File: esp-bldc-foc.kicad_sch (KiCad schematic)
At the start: 8 parts, among them J10 UART, J7 A, J8 B, J9 C

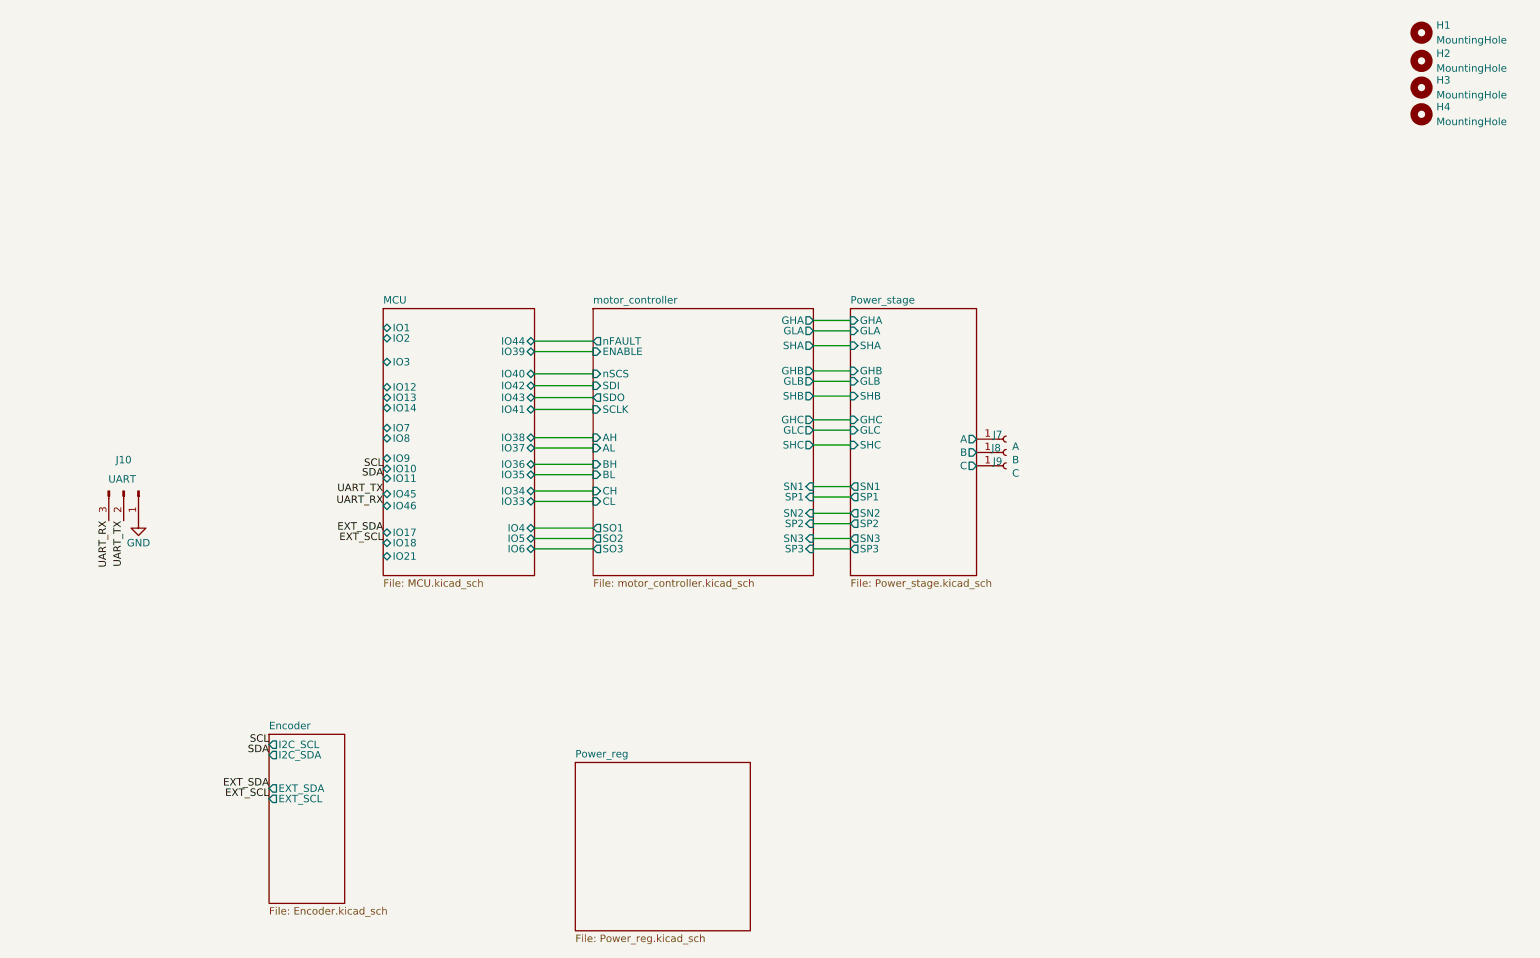
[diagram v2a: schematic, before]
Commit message: init routing done
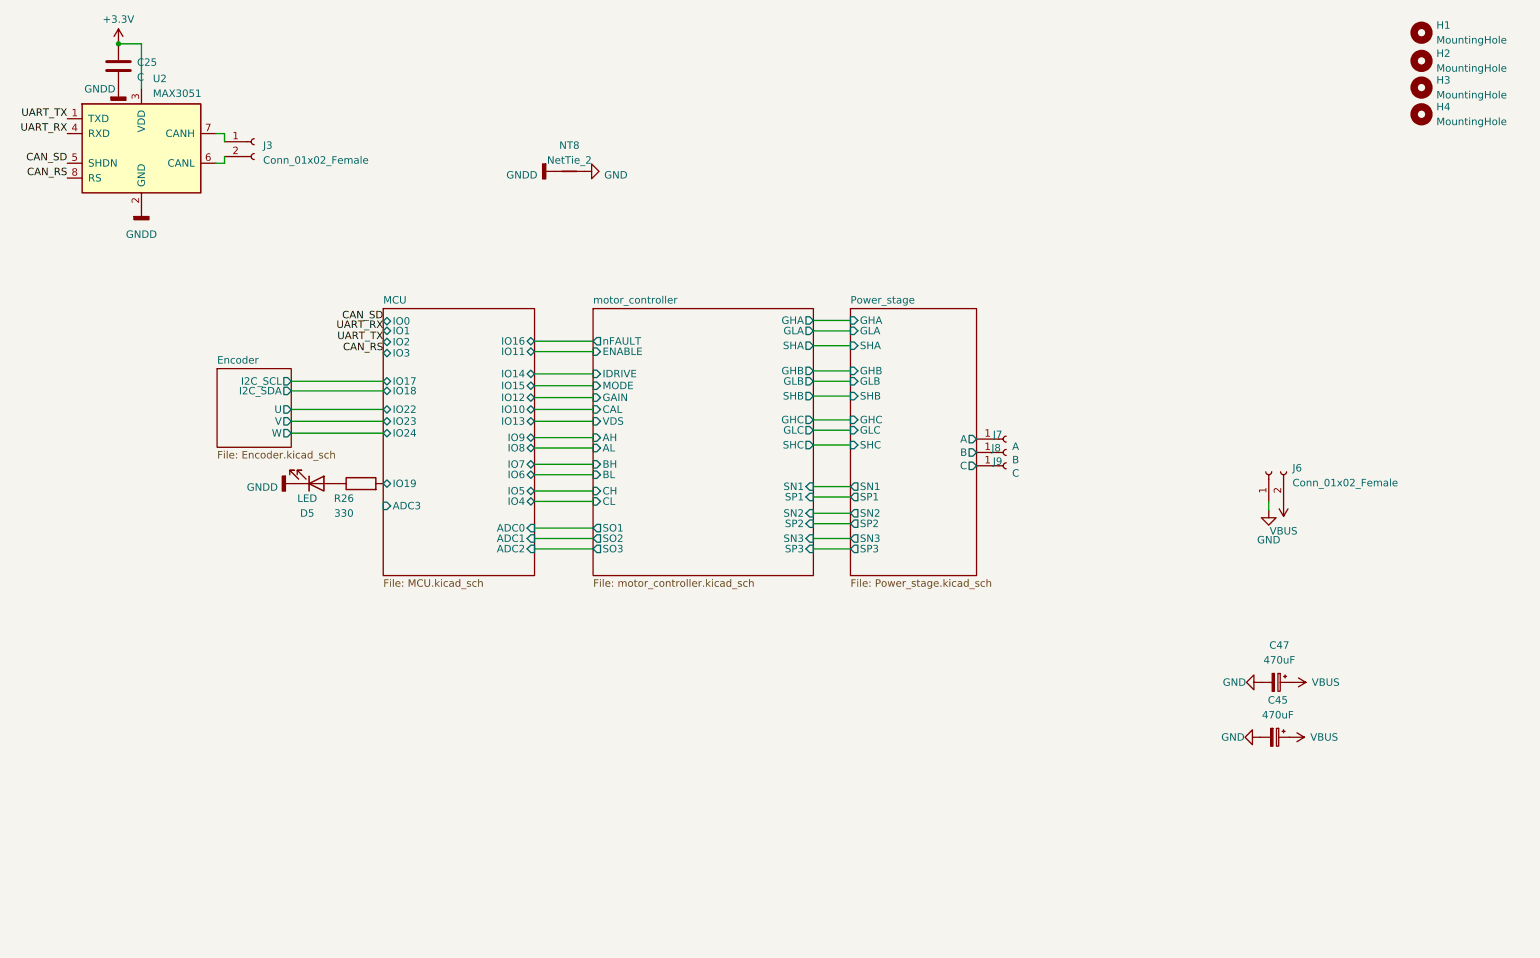
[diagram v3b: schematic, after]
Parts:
- removed J10: UART, Connector_JST:JST_PH_B3B-PH-K_1x03_P2.00mm_Vertical, symbol Connector:Conn_01x03_Male
- added C25: C, Capacitor_SMD:C_0402_1005Metric, symbol Device:C
- added C45, C47: 470uF, Capacitor_SMD:CP_Elec_10x10, symbol Device:C_Polarized_Small
- added D5: LED, LED_SMD:LED_0603_1608Metric, symbol Device:LED
- added J3: Conn_01x02_Female, Connector_Molex:Molex_CLIK-Mate_502443-0270_1x02-1MP_P2.00mm_Vertical, symbol Connector:Conn_01x02_Female
- added J6: Conn_01x02_Female, Connector_AMASS:AMASS_XT30U-F_1x02_P5.0mm_Vertical, symbol Connector:Conn_01x02_Female
- added NT8: NetTie_2, NetTie:NetTie-2_SMD_Pad2.0mm, symbol Device:NetTie_2
- added R26: 330, Resistor_SMD:R_0402_1005Metric, symbol Device:R
- added U2: MAX3051, Package_SO:SOIC-8_3.9x4.9mm_P1.27mm, symbol Interface_UART:MAX3051
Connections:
- net GND: now also C45.2, C47.2, J6.1 (Pin_1), NT8.2
- net UART_RX: now also U2.4 (RXD)
- net UART_TX: now also U2.1 (TXD)
- new net: D5.2 (A), R26.1
- new net: J3.2 (Pin_2), U2.6 (CANL)
- new net: J3.1 (Pin_1), U2.7 (CANH)
- new net +3.3V: C25.1, U2.3 (VDD)
- new net CAN_RS: U2.8 (RS)
- new net CAN_SD: U2.5 (SHDN)
- new net GNDD: C25.2, D5.1 (K), NT8.1, U2.2 (GND)
- new net MCU/IO19: R26.2
- new net VBUS: C45.1, C47.1, J6.2 (Pin_2)
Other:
- removed sheet Power_reg
- sheet Encoder ports: added U, V, W; removed EXT_SCL, EXT_SDA
- sheet MCU ports: added ADC0, ADC1, ADC2, ADC3, IO0, IO15, IO16, IO19, IO22, IO23, IO24; removed IO21, IO33, IO34, IO35, IO36, IO37, IO38, IO39, IO40, IO41, IO42, IO43, IO44, IO45, IO46
- sheet motor_controller ports: added CAL, GAIN, IDRIVE, MODE, VDS; removed SCLK, SDI, SDO, nSCS

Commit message: designed
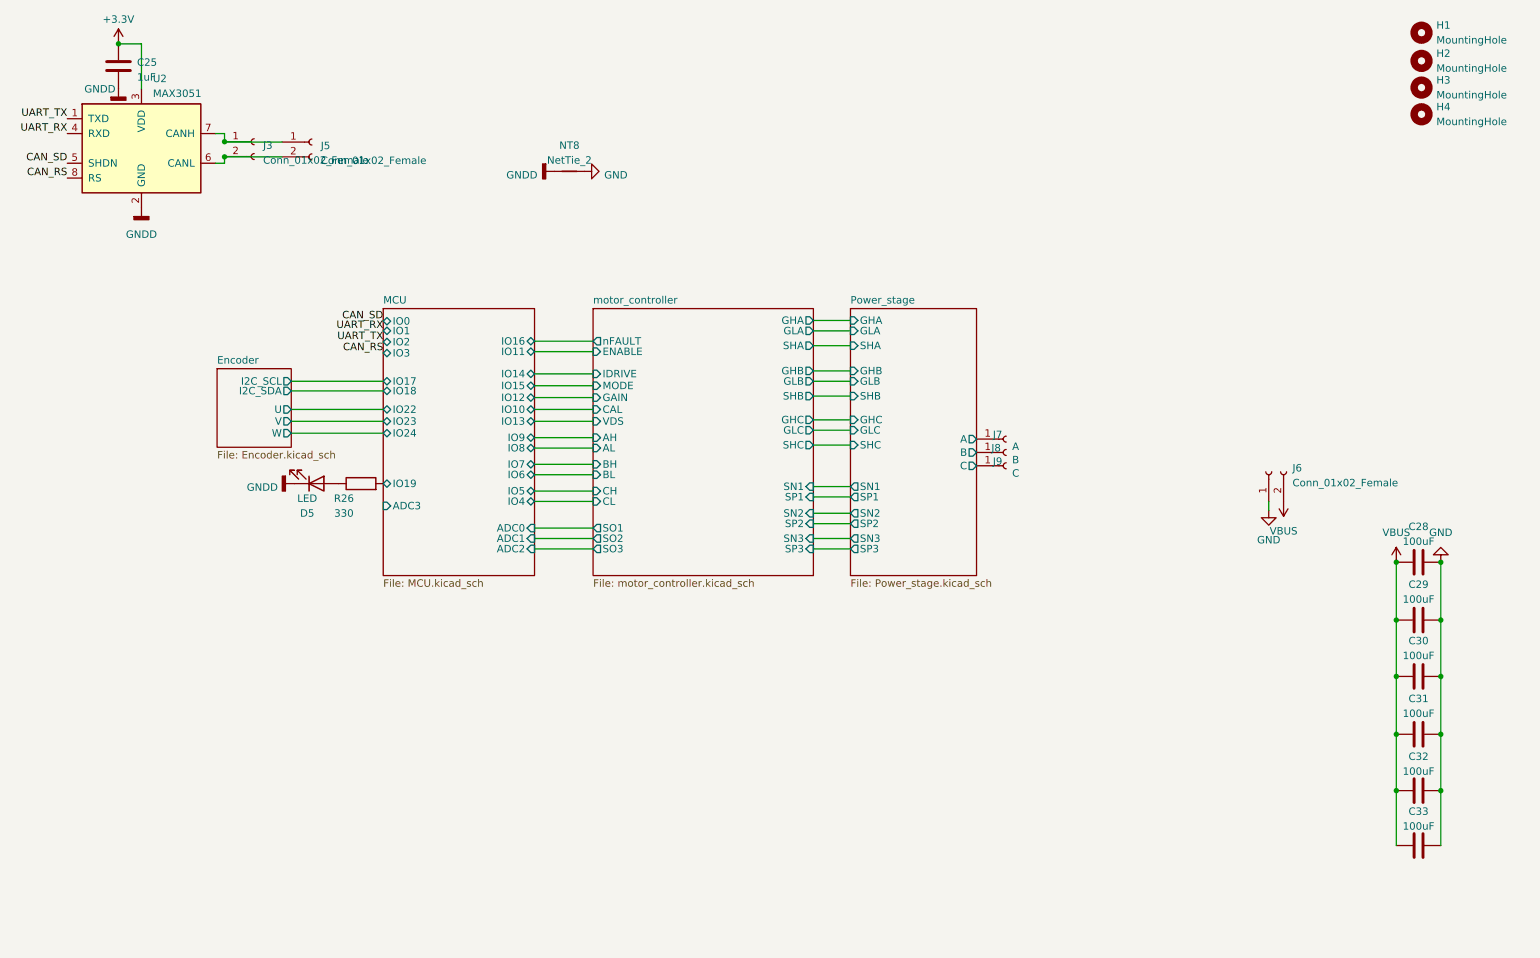
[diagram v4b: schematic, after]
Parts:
- removed C45, C47: 470uF, Capacitor_SMD:CP_Elec_10x10, symbol Device:C_Polarized_Small
- added C28, C29, C30, C31, C32, C33: 100uF, Capacitor_SMD:C_1206_3216Metric, symbol Device:C
- added J5: Conn_01x02_Female, Connector_Molex:Molex_CLIK-Mate_502443-0270_1x02-1MP_P2.00mm_Vertical, symbol Connector:Conn_01x02_Female
- C25: value C -> 1uF
- H1, H2, H3, H4, J7, J8, J9: now left out of the parts list
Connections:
- net GND: now also C28.2, C29.2, C30.2, C31.2, C32.2, C33.2
- net VBUS: now also C28.1, C29.1, C30.1, C31.1, C32.1, C33.1
- net at J3.2 (Pin_2), U2.6 (CANL): now also J5.2 (Pin_2)
- net at J3.1 (Pin_1), U2.7 (CANH): now also J5.1 (Pin_1)
